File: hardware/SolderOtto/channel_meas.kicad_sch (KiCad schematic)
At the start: 62 parts, among them Q901 BC847A, Q902 BC858B, Q903 BC847A, U901 OPA2206, U902 LM358B, U903 74hc4053, U905 OPA206

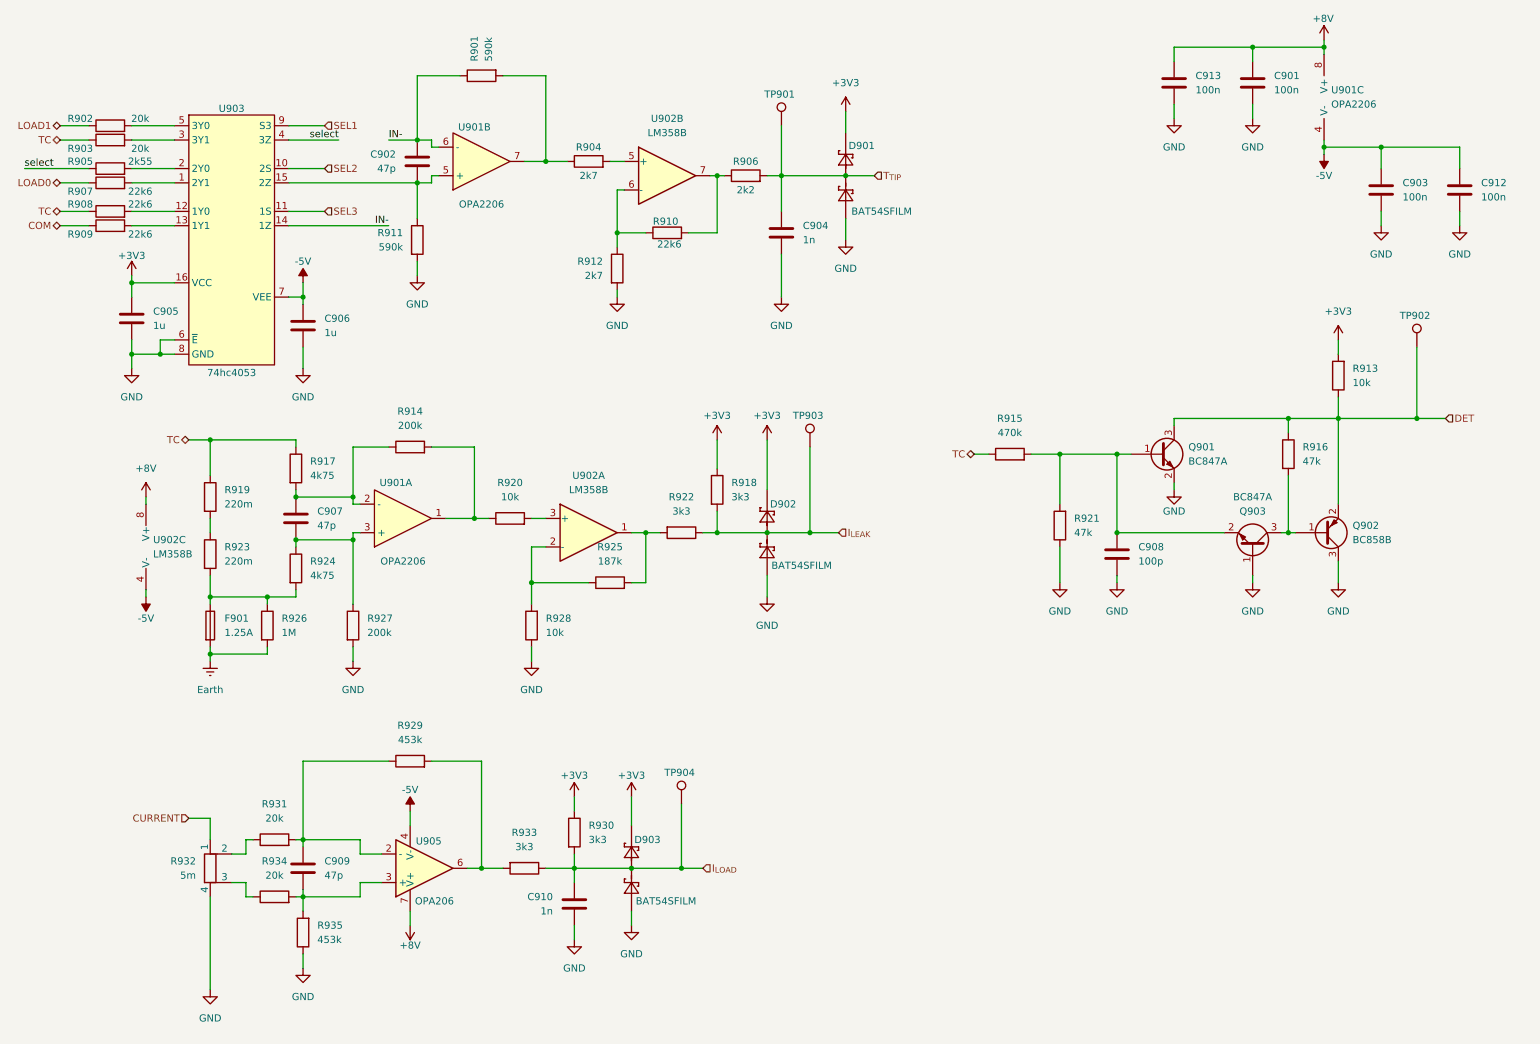
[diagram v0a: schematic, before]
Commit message: save work
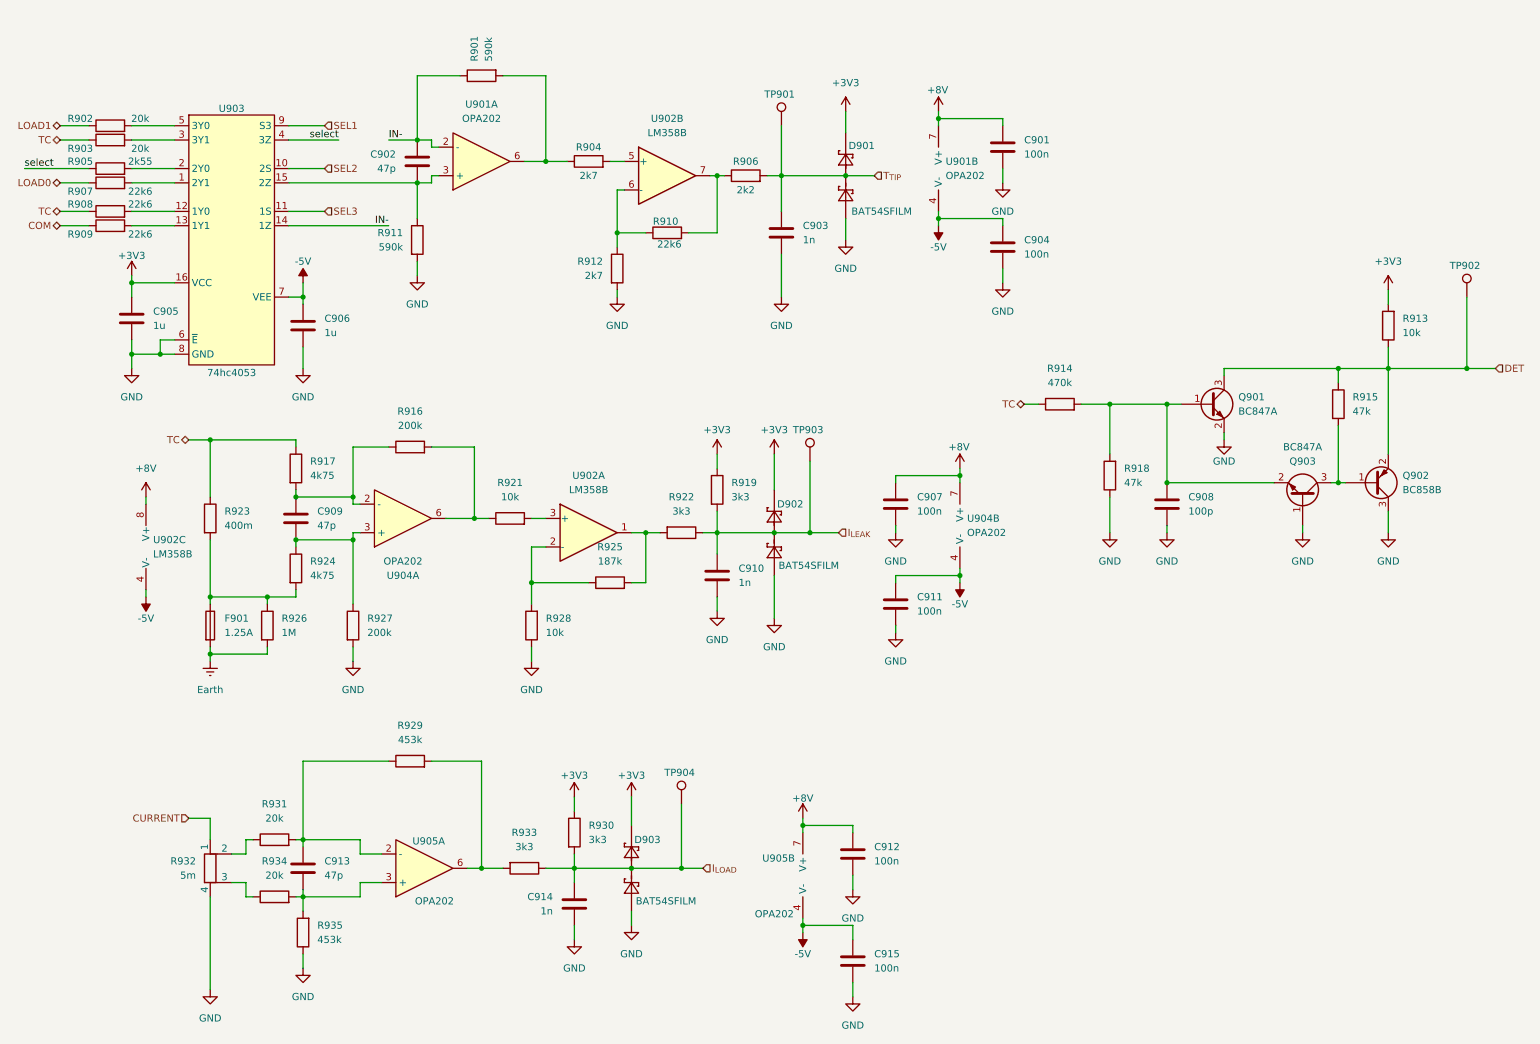
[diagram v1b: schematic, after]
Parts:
- removed R919: 220m, Resistor_SMD:R_0603_1608Metric, symbol Device:R
- removed U901: OPA2206, Package_SO:VSSOP-8_3x3mm_P0.65mm, symbol mylib_ic:OPA2206
- added C904, C907: 100n, Capacitor_SMD:C_0603_1608Metric, symbol Device:C
- added C910: 1n, Capacitor_SMD:C_0603_1608Metric, symbol Device:C
- added U901, U904: OPA202, Package_SO:VSSOP-8_3x3mm_P0.65mm, symbol mylib_ic:OPA206
- added unit 2 of U905
- R923: value 220m -> 400m; footprint Resistor_SMD:R_0603_1608Metric -> Resistor_SMD:R_1206_3216Metric; Digikey P.22AJCT-ND -> 283-MFHA1206R4000FCCT-ND
- U905: value OPA206 -> OPA202; Field5 (none) -> 296-OPA202IDGKRCT-ND
- renumbered C904 to C903, C907 to C909, C912 to C911, C913 to C912, C909 to C913, C910 to C914, C903 to C915, R915 to R914, R916 to R915, R914 to R916, R921 to R918, R918 to R919, R920 to R921
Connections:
- net +8V: now also C907.1, U901.7 (V+), U904.7 (V+), U905.7 (V+); no longer U905.7 (V+)
- net -5V: now also C904.1, U901.4 (V-), U904.4 (V-), U905.4 (V-); no longer U905.4 (V-)
- net GND: now also C904.2, C907.2, C910.2
- net IN-: now also U901.2 (-)
- net I_{LEAK}: now also C910.1
- net TC: now also R923.1
- net at C909.1, R916.1, R917.2: now also U904.2 (-)
- net at R916.2, R921.1: now also U904.6
- net at C909.2, R924.1, R927.1: now also U904.3 (+)
- net at C902.2, R911.1, U903.15 (2Z): now also U901.3 (+)
- net at R901.2, R904.1: now also U901.6
- new net: U904.1 (NC), U904.5 (NC), U904.8 (NC)
- new net: U901.1 (NC), U901.5 (NC), U901.8 (NC)
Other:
- moved on the sheet: C901, C908, C911, C912, C915, D902, Q901, Q902, Q903, R913, R914, R915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
